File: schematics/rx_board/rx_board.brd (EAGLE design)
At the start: 27 x 40 mm, 15 parts, among them U1 SI4463-C2A-GM, X2 SMA

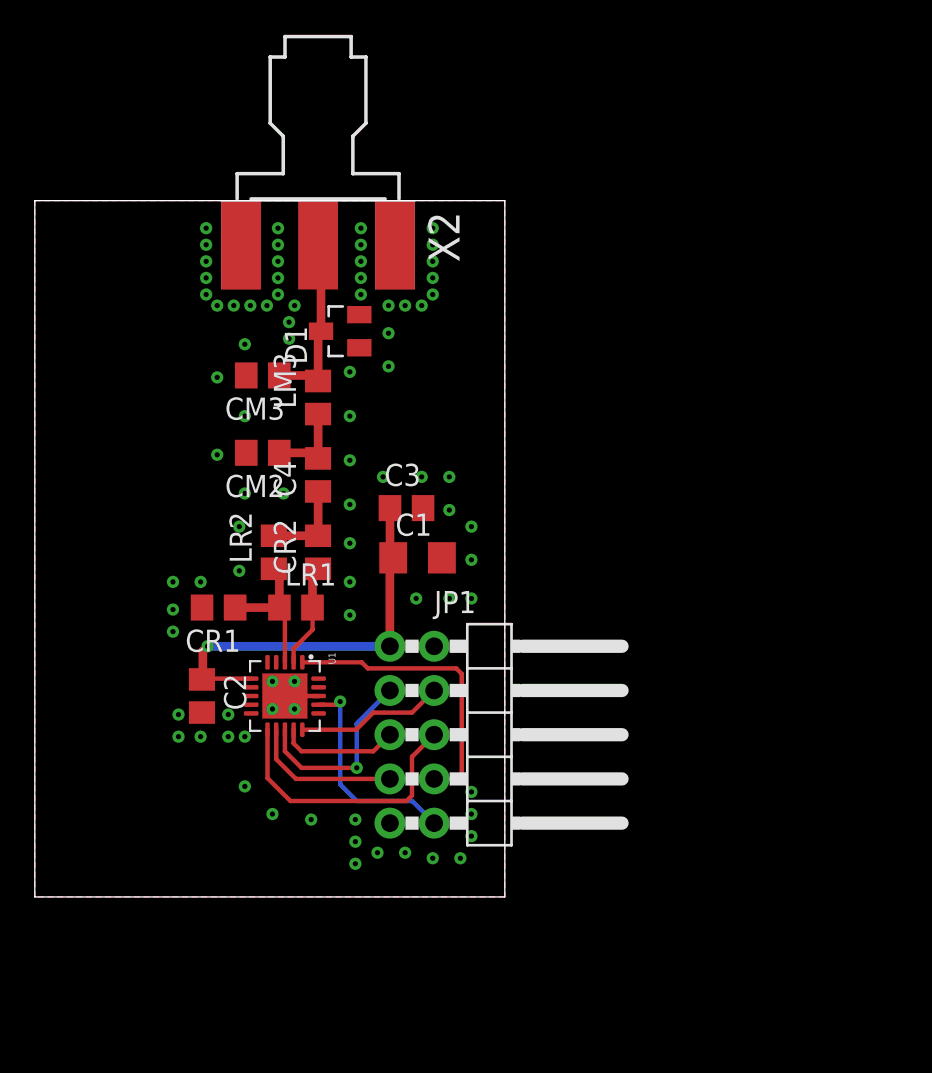
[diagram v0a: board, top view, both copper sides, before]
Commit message: Add files via upload
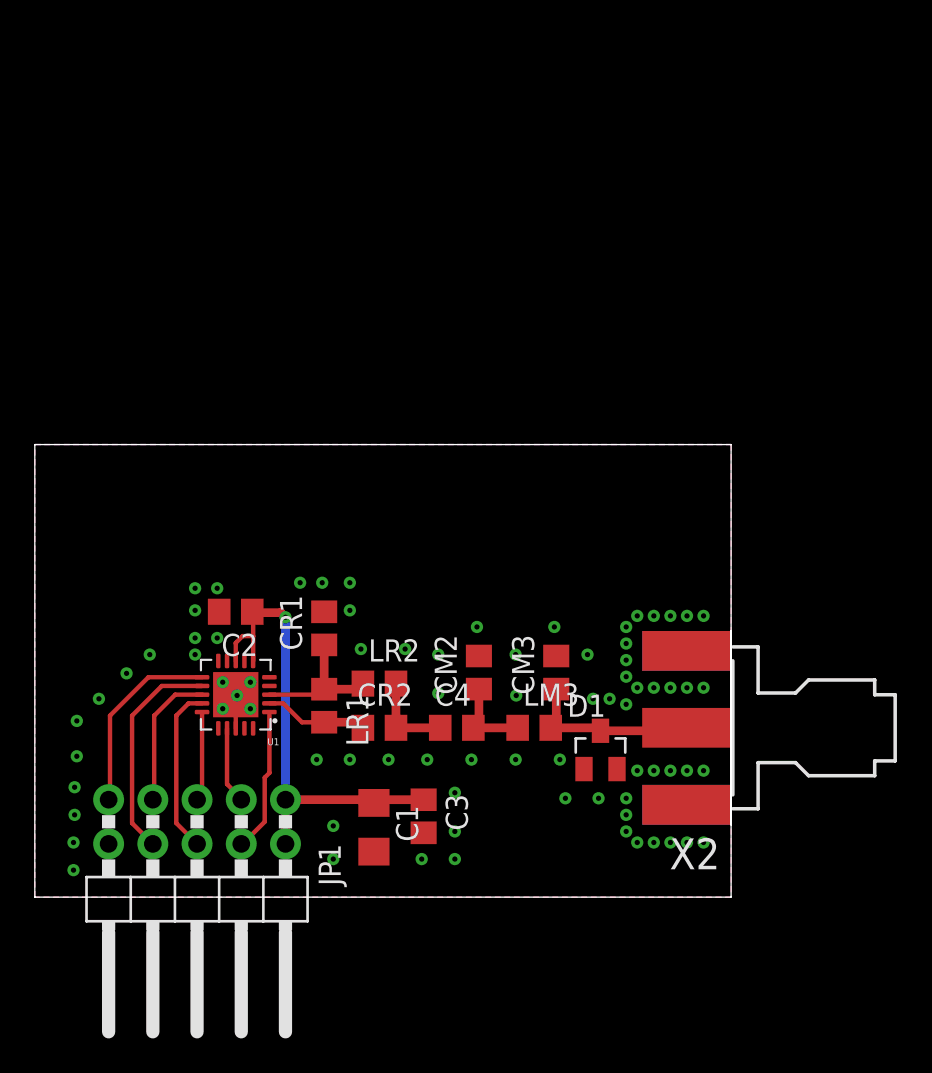
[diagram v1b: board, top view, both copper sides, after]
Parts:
- moved X2 38.5 mm to (40.0, 9.71), turned to 180 degrees
- moved D1 28.3 mm to (32.5, 8.45), turned to 0 degrees
- moved CM3 24.0 mm to (30.0, 12.9), turned to 90 degrees
- moved LM3 22.7 mm to (28.7, 9.71), turned to 0 degrees
- moved JP1 20.1 mm to (9.32, -0.76), turned to 180 degrees
- moved C3 17.7 mm to (22.3, 4.63), turned to 270 degrees
- moved CM2 17.7 mm to (25.5, 12.9), turned to 90 degrees
- moved C4 16.6 mm to (24.2, 9.71), turned to 0 degrees
- moved C1 15.7 mm to (19.5, 4.00), turned to 270 degrees
- moved CR2 10.7 mm to (19.8, 9.71), turned to 0 degrees
- moved LR2 9.68 mm to (19.8, 12.3), turned to 0 degrees
- moved CR1 6.18 mm to (16.6, 15.4), turned to 90 degrees
- moved LR1 5.87 mm to (16.6, 11.0), turned to 270 degrees
- moved C2 5.21 mm to (11.5, 16.4), turned to 180 degrees
- moved U1 2.83 mm to (11.5, 11.6), turned to 180 degrees
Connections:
- net CLK_REF: now also JP1.3; no longer JP1.10
- net GND: now also JP1.10; no longer JP1.9
- net NIRQ: now also JP1.9; no longer JP1.6
- net NSEL: now also JP1.5; no longer JP1.4
- net SCLK: now also JP1.8; no longer JP1.7
- net SDI: now also JP1.6; no longer JP1.5
- net SDN: now also JP1.4; no longer JP1.8
- net SDO: now also JP1.7; no longer JP1.3
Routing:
- net SDN: track 16.9 -> 8.29 mm
- net CLK_REF: track 12.4 -> 4.44 mm, vias 1 -> 0
- net NIRQ: track 15.8 -> 11.1 mm
- net SCLK: track 8.70 -> 12.6 mm
- net NSEL: track 8.51 -> 5.15 mm
- net SDO: track 11.0 -> 8.11 mm, vias 1 -> 0
- net SDI: track 6.90 -> 9.63 mm
- net +3V3: track 25.9 -> 28.1 mm
- net GND: vias 83 -> 78
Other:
- board size 27 x 40 mm -> 40 x 26 mm
